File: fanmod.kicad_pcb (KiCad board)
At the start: 2 copper layers, 15 x 15 mm, 6 parts, among them J1 FAN_IN, J2 FAN_OUT, J4 COMM

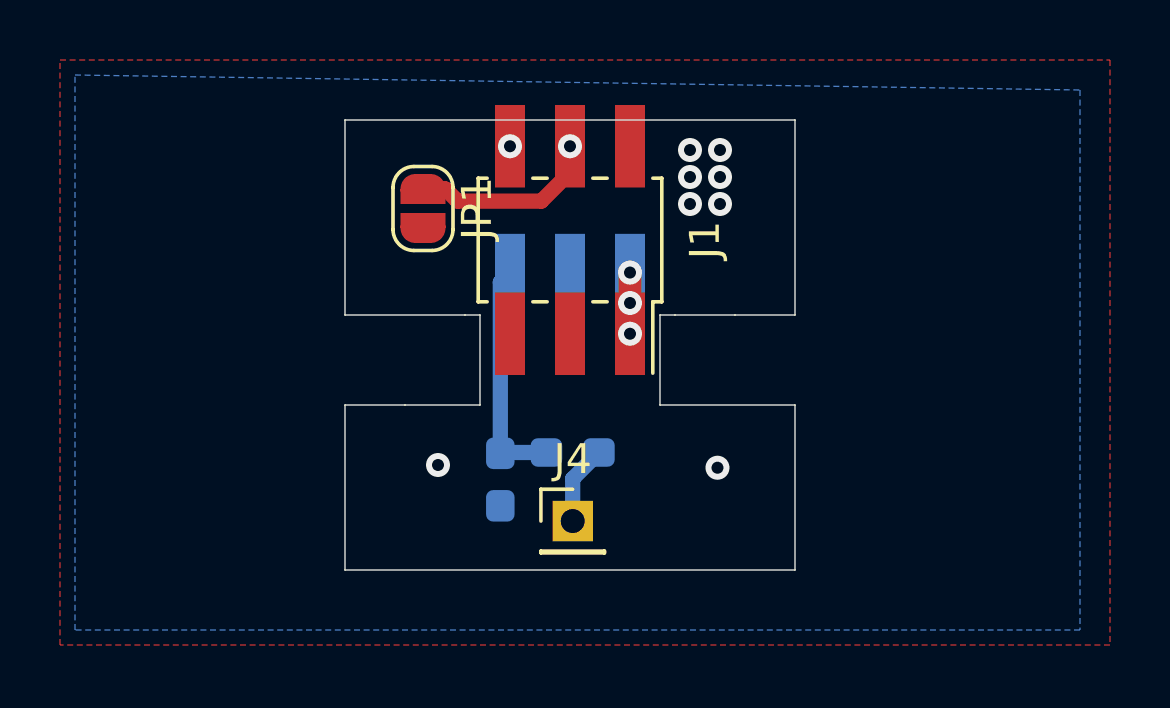
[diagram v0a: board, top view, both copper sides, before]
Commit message: First commit
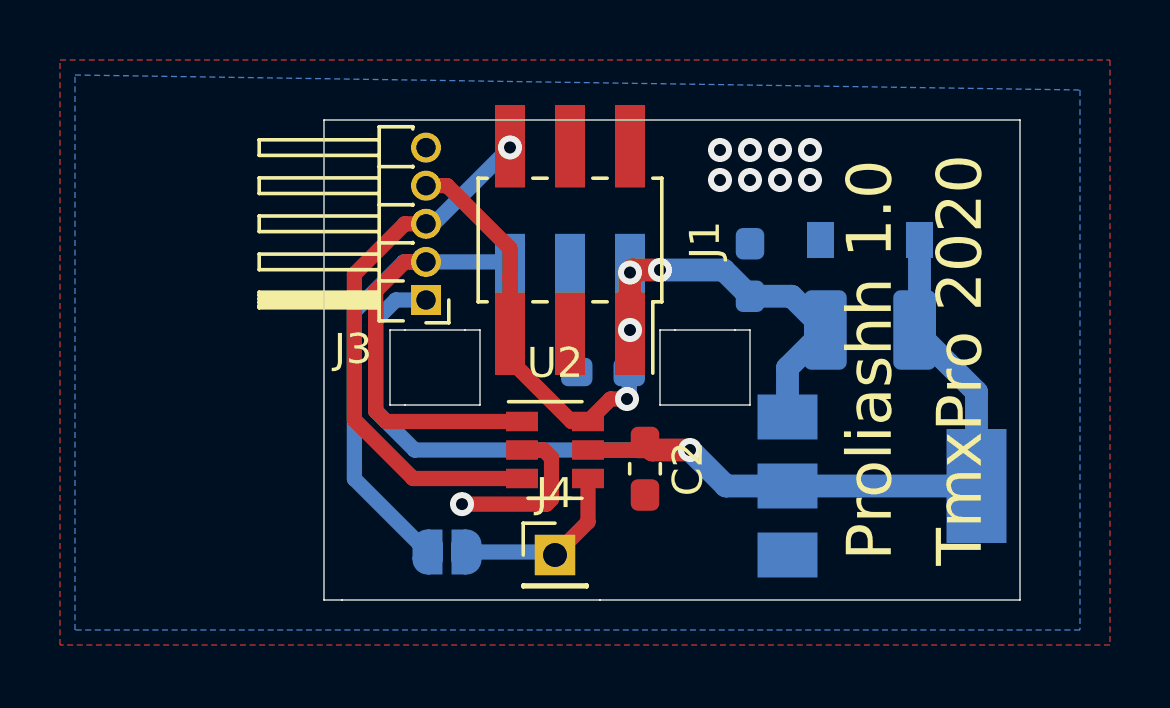
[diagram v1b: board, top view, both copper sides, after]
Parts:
- removed R2: 2k, Resistor_SMD:R_0603_1608Metric_Pad1.05x0.95mm_HandSolder
- added C1: 10u, Capacitor_SMD:C_0603_1608Metric_Pad1.05x0.95mm_HandSolder, B.Cu at (91.0, 23.0)
- added C2: 10u, Capacitor_SMD:C_0603_1608Metric_Pad1.05x0.95mm_HandSolder, F.Cu at (87.5, 29.6)
- added C3: C, Capacitor_SMD:C_0603_1608Metric_Pad1.05x0.95mm_HandSolder, B.Cu at (86.1, 26.4)
- added D1: 3.3V, Diode_SMD:D_SOD-123, B.Cu at (95.0, 22.0)
- added J3: Conn_01x05, Connector_PinHeader_1.27mm:PinHeader_1x05_P1.27mm_Horizontal, F.Cu at (80.2, 24.0)
- added U1: LM1117-3.3, Package_TO_SOT_SMD:SOT-223-3_TabPin2, B.Cu at (95.4, 30.2)
- added U2: ATtiny10-TS, Package_TO_SOT_SMD:SOT-23-6, F.Cu at (84.5, 29.0)
- JP1: value BYPASS -> PROXY; moved to B.Cu
- R1: value 1k -> 200R 0.5W; footprint Resistor_SMD:R_0603_1608Metric_Pad1.05x0.95mm_HandSolder -> Resistor_SMD:R_1210_3225Metric_Pad1.42x2.65mm_HandSolder
- moved JP1 11.5 mm to (80.9, 32.4), turned to 180 degrees
- moved R1 10.7 mm to (95.0, 25.0), turned to 0 degrees
- moved J4 1.28 mm to (84.5, 32.5)
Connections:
- net ROTATION_DETECT renamed PROG_CLK
- J1 pad 2: GND -> GROUND_LOOP
- J1 pad 5: (no net) -> MCU_RESET
- J2 pad 2: GND -> GROUND_LOOP
- J2 pad 4: GROUND_LOOP -> (no net)
- J2 pad 5: Net-(J2-Pad5) -> PROG_DATA
- J4 pad 1: Net-(J4-Pad1) -> COMM
- JP1 pad 1: GROUND_LOOP -> COMM
- JP1 pad 2: GND -> PROG_DATA
- R1 pad 1: Net-(J4-Pad1) -> +12V
- R1 pad 2: Net-(J2-Pad5) -> +3V3
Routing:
- net +3V3: track 0.00 -> 38.8 mm, vias 0 -> 1
- net PROG_DATA: track 0.00 -> 26.2 mm
- net PROG_CLK: track 0.04 -> 18.2 mm
- net MCU_RESET: track 0.00 -> 13.4 mm, vias 0 -> 1
- net +12V: track 4.08 -> 12.8 mm
- net Net-(J2-Pad5): track 7.71 -> 0.00 mm
- net COMM: track 0.00 -> 6.00 mm
- net Net-(J4-Pad1): track 2.65 -> 0.00 mm
- net GROUND_LOOP: track 6.34 -> 5.52 mm, vias 1 -> 9
- net GND: vias 8 -> 0
- added copper zone on B.Cu, net GROUND_LOOP
- added copper zone on F.Cu, net GROUND_LOOP
- removed copper zone on B.Cu, net GND
- removed copper zone on F.Cu, net GND
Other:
- board size 15 x 15 mm -> 23.2 x 16 mm
- board text added: "Proliashh 1.0"
- board text added: "TmxPro 2020"
